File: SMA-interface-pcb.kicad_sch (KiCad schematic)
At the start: 15 parts, among them J1 Conn_Coaxial, J2 Conn_Coaxial, J3 Conn_01x02_Pin, J4 USB_A_Stacked, J5 Conn_01x02_Pin, Q1 AO3400A, Q2 AO3400A, U1 EL817, U2 EL817

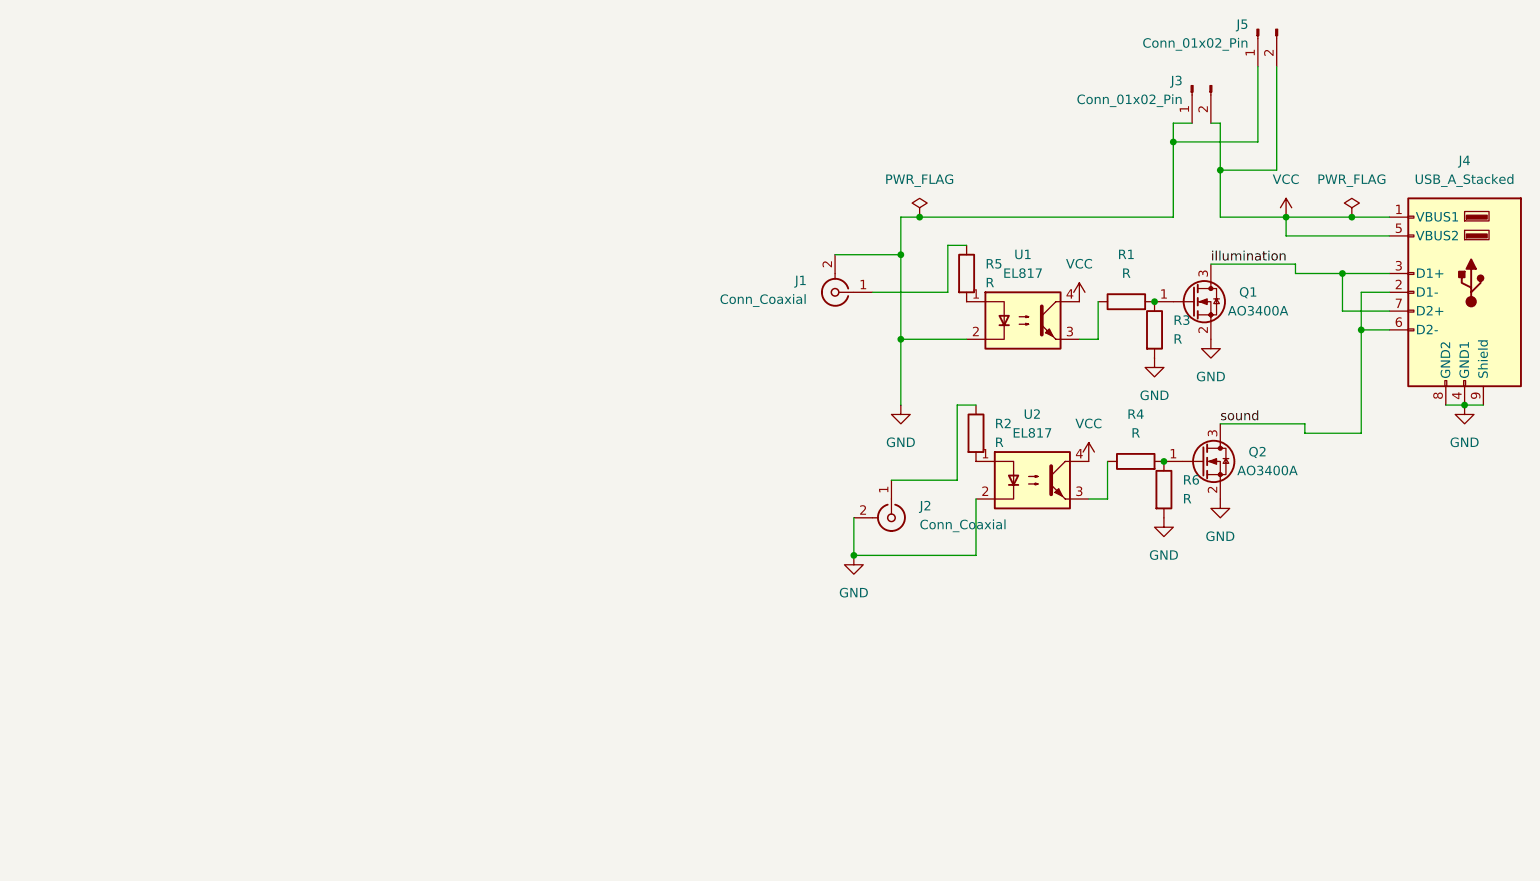
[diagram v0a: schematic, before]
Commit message: updated active buzzer system
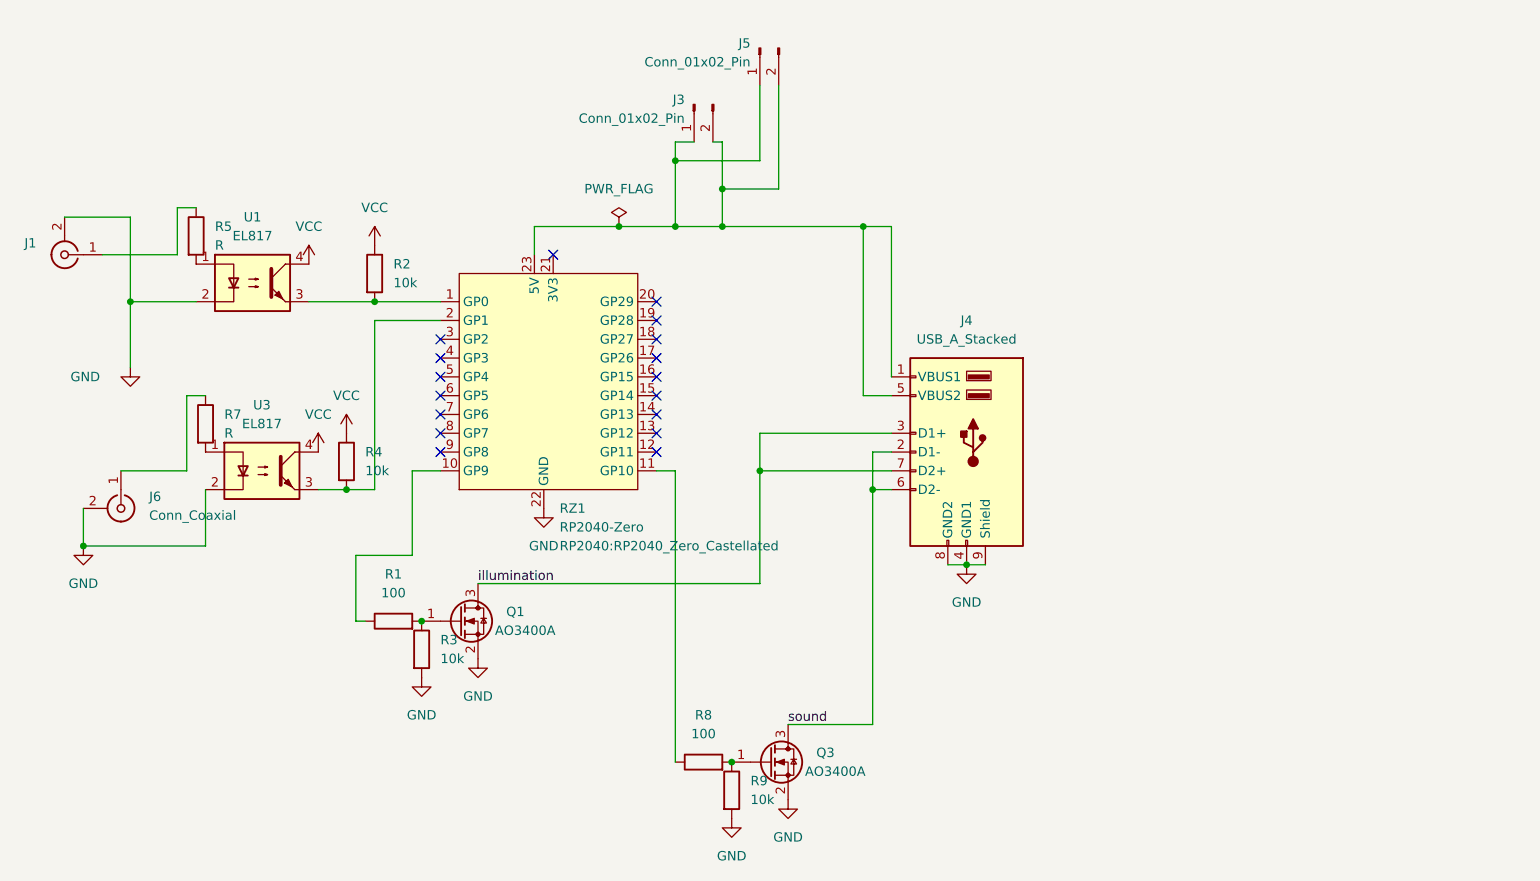
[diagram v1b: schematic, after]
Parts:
- removed J2: Conn_Coaxial, Connector_Coaxial:SMA_Amphenol_901-143_Horizontal, symbol Connector:Conn_Coaxial
- removed Q2: AO3400A, Package_TO_SOT_SMD:SOT-23, symbol Transistor_FET:AO3400A
- removed R6: R, Resistor_THT:R_Axial_DIN0207_L6.3mm_D2.5mm_P2.54mm_Vertical, symbol Device:R
- removed U2: EL817, Package_DIP:DIP-4_W7.62mm_SMDSocket_SmallPads, symbol Isolator:EL817
- added J6: Conn_Coaxial, Connector_Coaxial:SMA_Amphenol_901-143_Horizontal, symbol Connector:Conn_Coaxial
- added Q3: AO3400A, Package_TO_SOT_SMD:SOT-23, symbol Transistor_FET:AO3400A
- added R7: R, Resistor_THT:R_Axial_DIN0207_L6.3mm_D2.5mm_P2.54mm_Vertical, symbol Device:R
- added R8: 100, Resistor_THT:R_Axial_DIN0207_L6.3mm_D2.5mm_P2.54mm_Vertical, symbol Device:R
- added R9: 10k, Resistor_THT:R_Axial_DIN0207_L6.3mm_D2.5mm_P2.54mm_Vertical, symbol Device:R
- added RZ1: RP2040-Zero, RP2040:RP2040_Zero_Castellated, symbol RP2040_symbol:RP2040-Zero
- added U3: EL817, Package_DIP:DIP-4_W7.62mm_SMDSocket_SmallPads, symbol Isolator:EL817
- R1: value R -> 100
- R2, R3, R4: value R -> 10k
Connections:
- net GND: now also J6.2 (Ext), Q3.2 (S), R9.2, RZ1.22 (GND), U3.2; no longer J3.1 (Pin_1), J5.1 (Pin_1)
- net VCC: now also R2.1, R4.1, U3.4; no longer J3.2 (Pin_2), J4.1 (VBUS1), J4.5 (VBUS2), J5.2 (Pin_2)
- net sound: now also Q3.3 (D)
- net at R4.2: now also RZ1.2 (GP1), U3.3
- net at U1.3: now also R2.2, RZ1.1 (GP0); no longer R1.1
- new net: R7.2, U3.1
- new net: R1.1, RZ1.10 (GP9)
- new net: J6.1 (In), R7.1
- new net: R8.1, RZ1.11 (GP10)
- new net: J3.1 (Pin_1), J3.2 (Pin_2), J4.1 (VBUS1), J4.5 (VBUS2), J5.1 (Pin_1), J5.2 (Pin_2), RZ1.23 (5V)
- new net: Q3.1 (G), R8.2, R9.1
- no-connect marks 0 -> 17
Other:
- moved on the sheet: J1, J3, J4, J5, Q1, R1, R3, R5, U1
